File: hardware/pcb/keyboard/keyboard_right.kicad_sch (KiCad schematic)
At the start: 35 parts, among them J1 SM04B-SRSS-TB, J2 PJ320D, J3 HRO_TYPE-C-31-M-12, J4 HRS_FH34SRJ-06S-0.5SH(50), SW29 PTS845, U3 PRTR5V0U2X, U4 XC6220B331MR-G, U5 STM32G431KBTx, U6 24FC01T-I/OT, Y1 8MHz 10pF

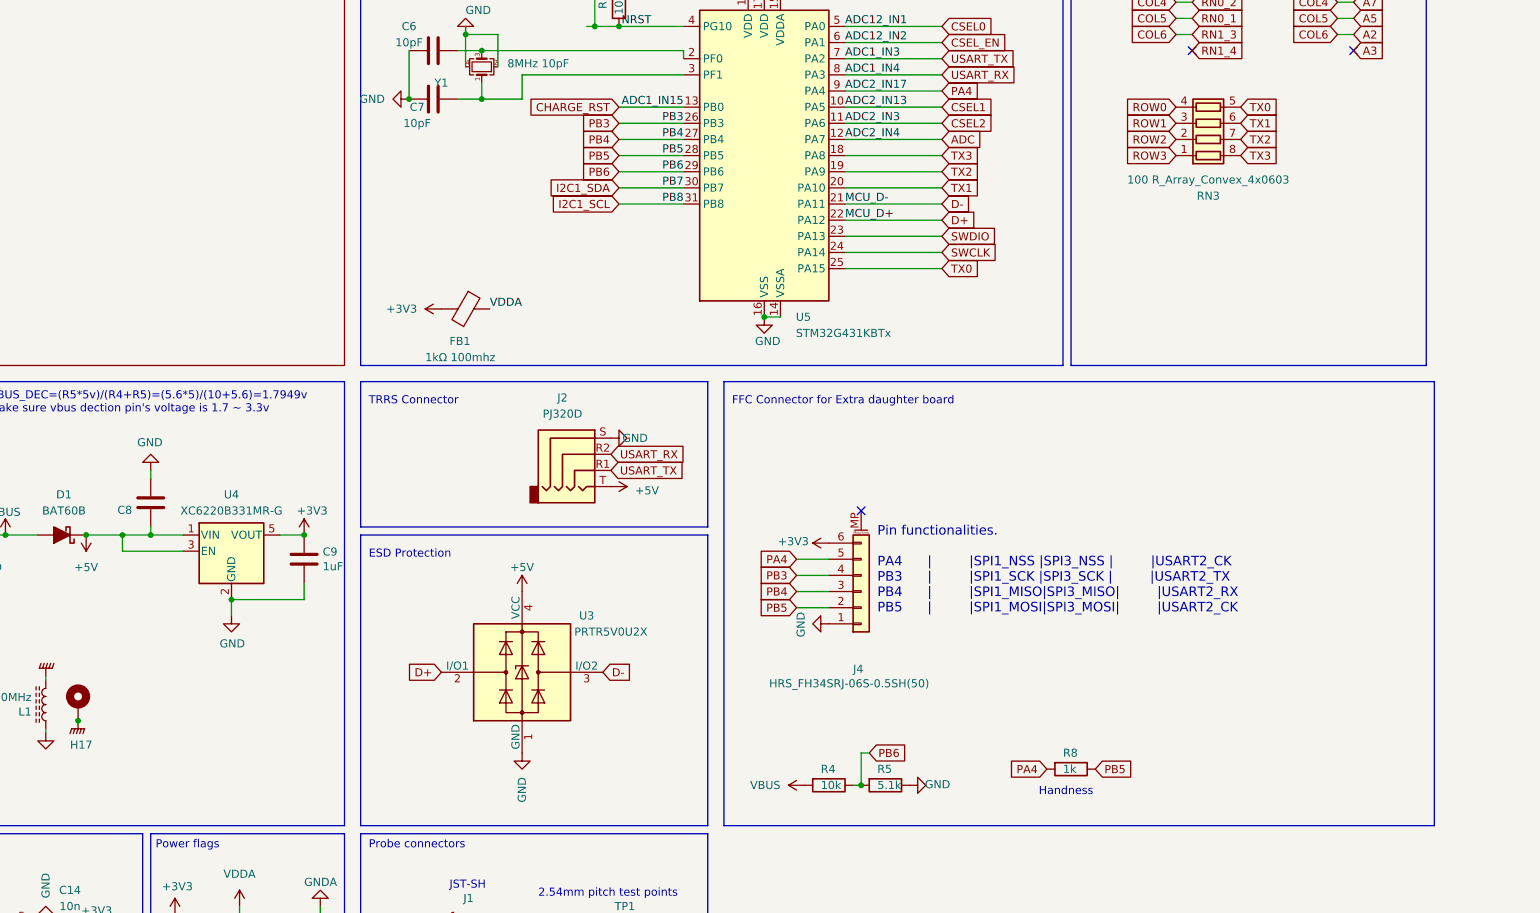
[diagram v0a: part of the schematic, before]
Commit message: stencil temp
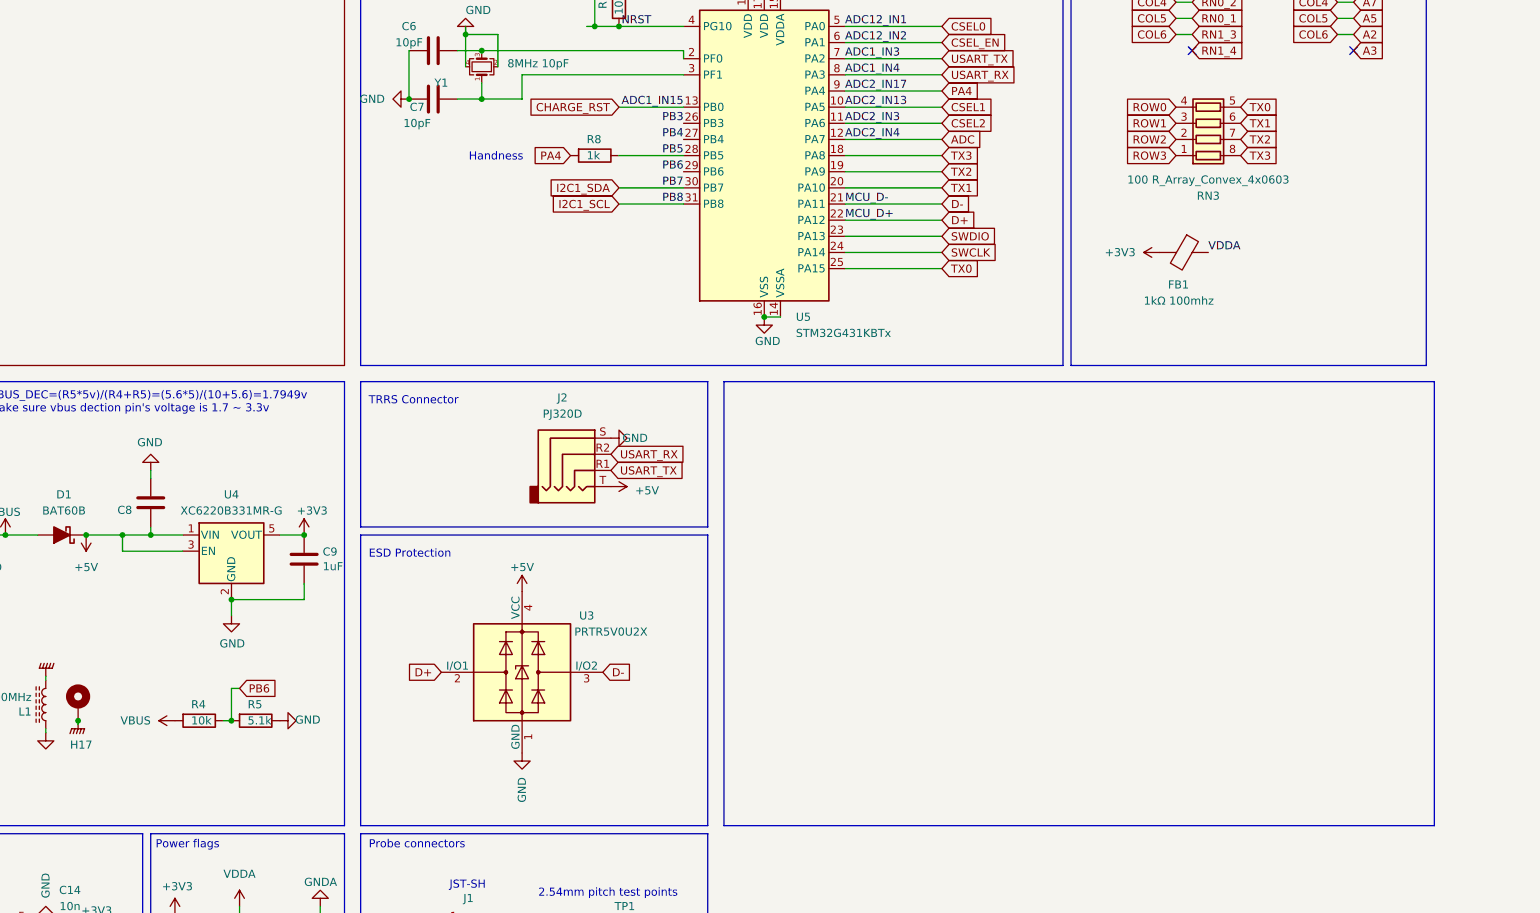
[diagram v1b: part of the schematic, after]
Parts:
- removed J4: HRS_FH34SRJ-06S-0.5SH(50), ec_parts:CONN6x1_FH34SRJ-6S-0.5SH50_HIR, symbol Connector_Generic_MountingPin:Conn_01x06_MountingPin
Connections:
- no-connect marks 10 -> 9
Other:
- note removed: "FFC Connector for Extra daughter board"
- note removed: "Pin functionalities. PA4 | |SPI1_NSS |SPI3_NSS | |USART2_CK PB3 | |SPI1_SCK |SPI3_SCK | |USART2_TX PB4 | |SPI1_MISO|SPI3_MISO| |USART2_RX PB5 | |SPI1_MOSI|SPI3_MOSI| |USART2_CK"
- moved on the sheet: FB1, R4, R5, R8

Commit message: Rev 2.1
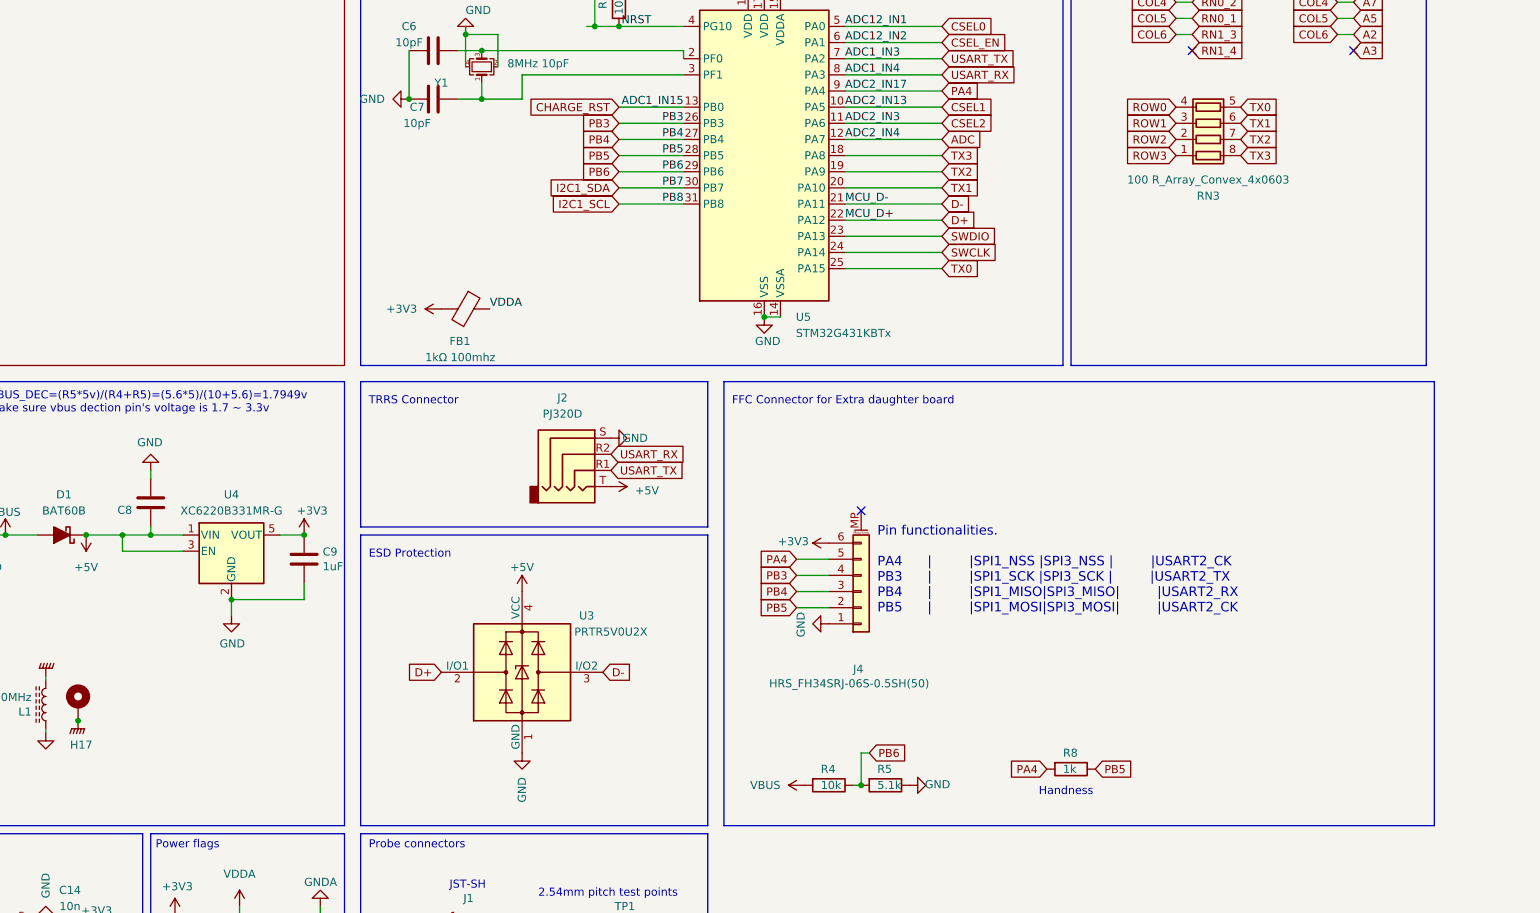
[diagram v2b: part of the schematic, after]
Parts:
- added J4: HRS_FH34SRJ-06S-0.5SH(50), ec_parts:CONN6x1_FH12S-6S-1SH55, symbol Connector_Generic_MountingPin:Conn_01x06_MountingPin
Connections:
- net +3V3: now also J4.6 (Pin_6)
- net GND: now also J4.1 (Pin_1)
- net PA4: now also J4.5 (Pin_5)
- net PB3: now also J4.4 (Pin_4)
- net PB4: now also J4.3 (Pin_3)
- net PB5: now also J4.2 (Pin_2)
- no-connect marks 9 -> 10
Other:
- note added: "FFC Connector for Extra daughter board"
- note added: "Pin functionalities. PA4 | |SPI1_NSS |SPI3_NSS | |USART2_CK PB3 | |SPI1_SCK |SPI3_SCK | |USART2_TX PB4 | |SPI1_MISO|SPI3_MISO| |USART2_RX PB5 | |SPI1_MOSI|SPI3_MOSI| |USART2_CK"
- moved on the sheet: FB1, R4, R5, R8
